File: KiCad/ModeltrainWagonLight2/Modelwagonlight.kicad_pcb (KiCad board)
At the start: 2 copper layers, 25 x 11 mm, 17 parts, among them J1 Conn_01x01, J2 Conn_01x01, J3 Conn_01x01, J4 Conn_01x01, U1 LP2951DR

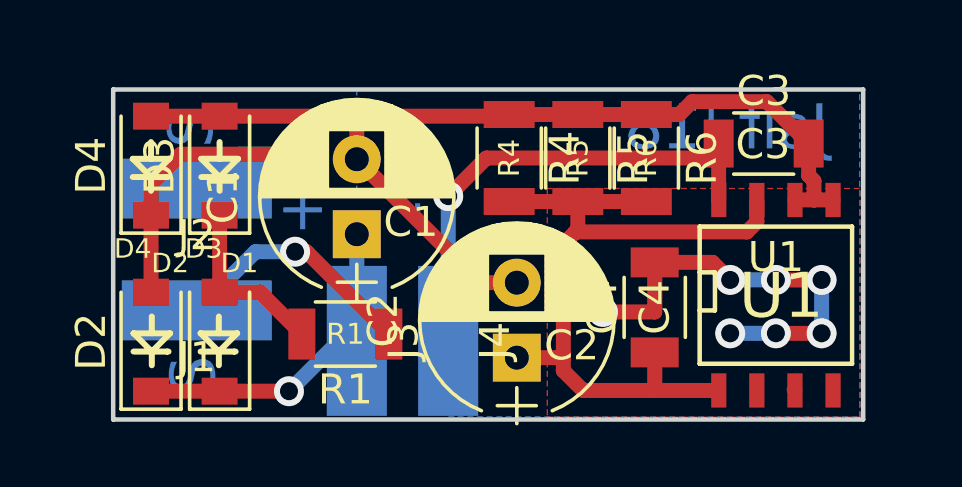
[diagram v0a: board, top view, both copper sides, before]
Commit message: Update om light2
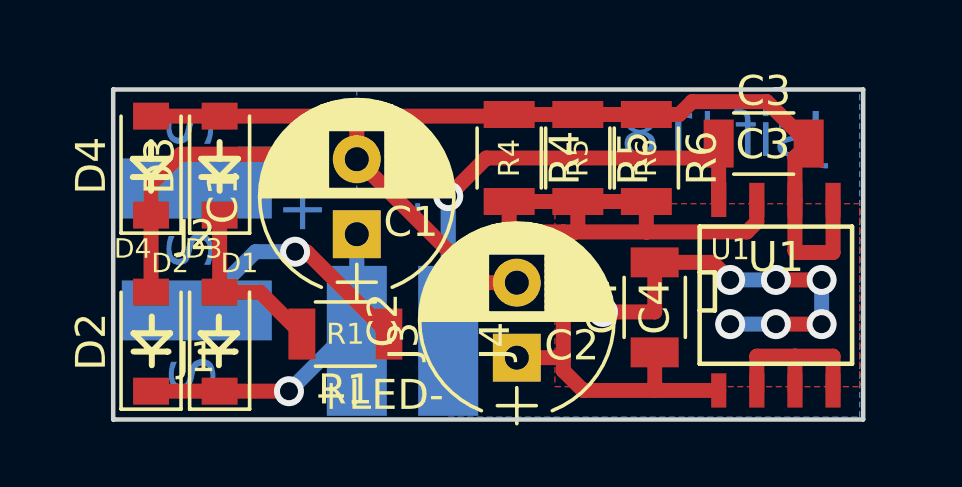
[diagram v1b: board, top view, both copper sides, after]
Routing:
- net Net-(C1-Pad2): track 48.5 -> 57.7 mm
- net Net-(C2-Pad1): track 26.0 -> 30.0 mm
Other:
- rule via_min_size: 0.4 -> 0.5
- board text added: "+LED-"
